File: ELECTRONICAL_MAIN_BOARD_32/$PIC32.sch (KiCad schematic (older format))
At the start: 42 parts, among them U1 PIC32MX795F512H

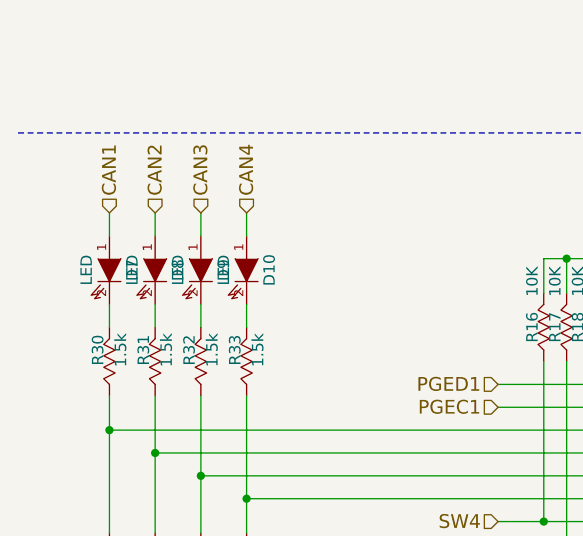
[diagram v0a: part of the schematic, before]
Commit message: mise a jour valeur
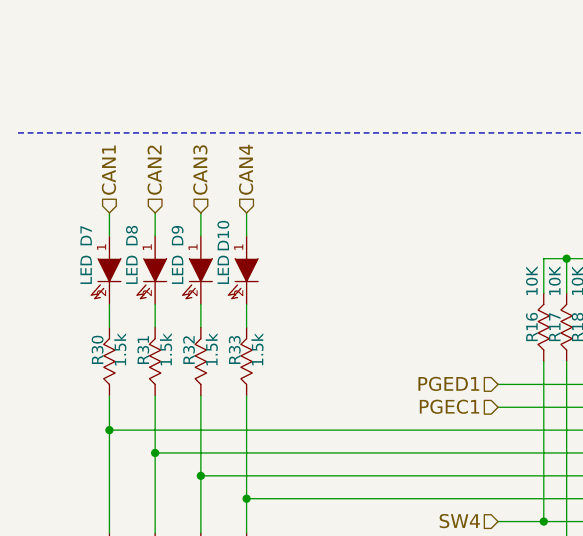
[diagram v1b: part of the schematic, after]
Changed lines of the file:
@@
-EESchema Schematic File Version 2  date 2012-08-29 22:13:25
+EESchema Schematic File Version 2  date 2012-08-29 22:32:21
 LIBS:conn
 LIBS:power
@@
 U 1 1 4FF078CE
 P 900 1750
-F 0 "D7" H 900 1850 50  0000 C CNN
+F 0 "D7" H 750 1650 50  0000 C CNN
 F 1 "LED" H 900 1650 50  0000 C CNN
 	1    900  1750
@@
 U 1 1 4FF078CD
 P 1100 1750
-F 0 "D8" H 1100 1850 50  0000 C CNN
+F 0 "D8" H 950 1650 50  0000 C CNN
 F 1 "LED" H 1100 1650 50  0000 C CNN
 	1    1100 1750
@@
 U 1 1 4FF078C6
 P 1500 1750
-F 0 "D10" H 1500 1850 50  0000 C CNN
+F 0 "D10" H 1350 1650 50  0000 C CNN
 F 1 "LED" H 1500 1650 50  0000 C CNN
 	1    1500 1750
@@
 U 1 1 4FF0781E
 P 1300 1750
-F 0 "D9" H 1300 1850 50  0000 C CNN
+F 0 "D9" H 1150 1650 50  0000 C CNN
 F 1 "LED" H 1300 1650 50  0000 C CNN
 	1    1300 1750
